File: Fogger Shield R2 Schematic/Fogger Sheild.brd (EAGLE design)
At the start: 53 x 47 mm, 23 parts, among them Q1 MOSFET-NCHANNELFQP30N06L, U1 ARDUINO_SHIELDLABEL

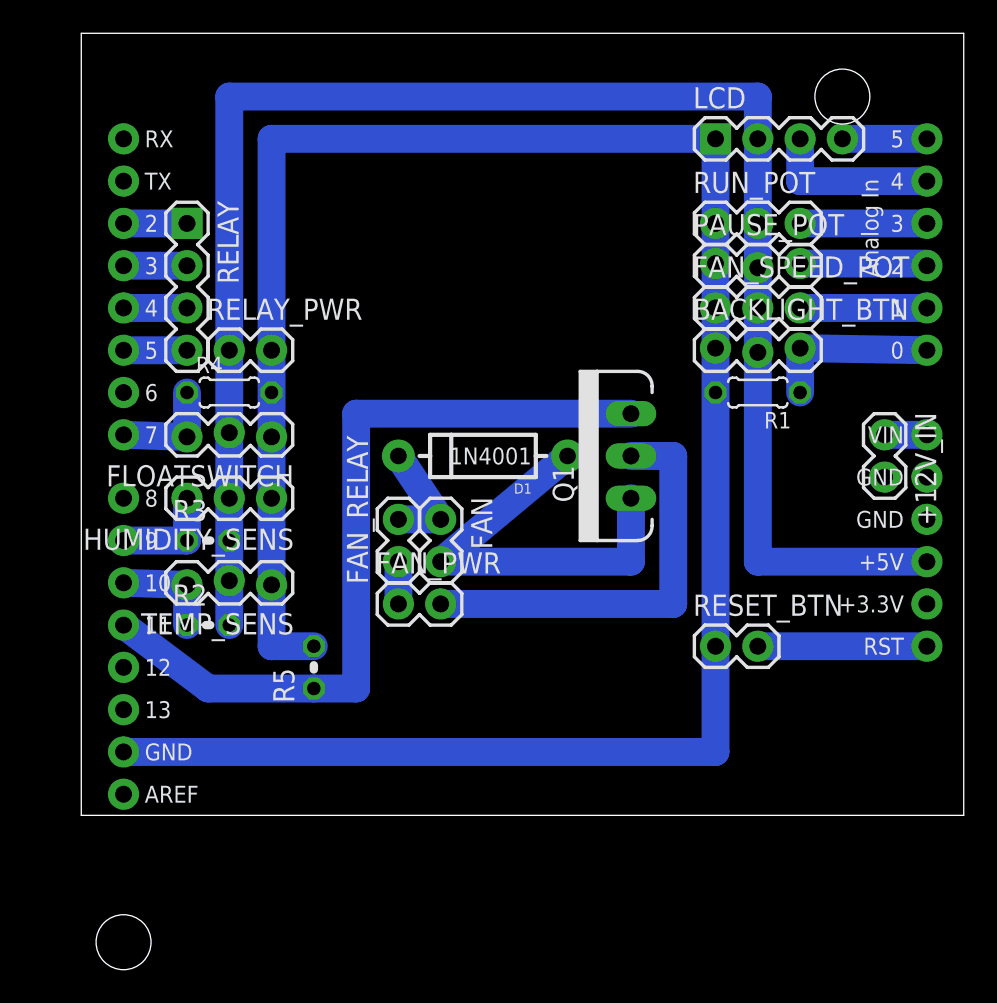
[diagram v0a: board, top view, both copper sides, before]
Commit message: Updated Schematic
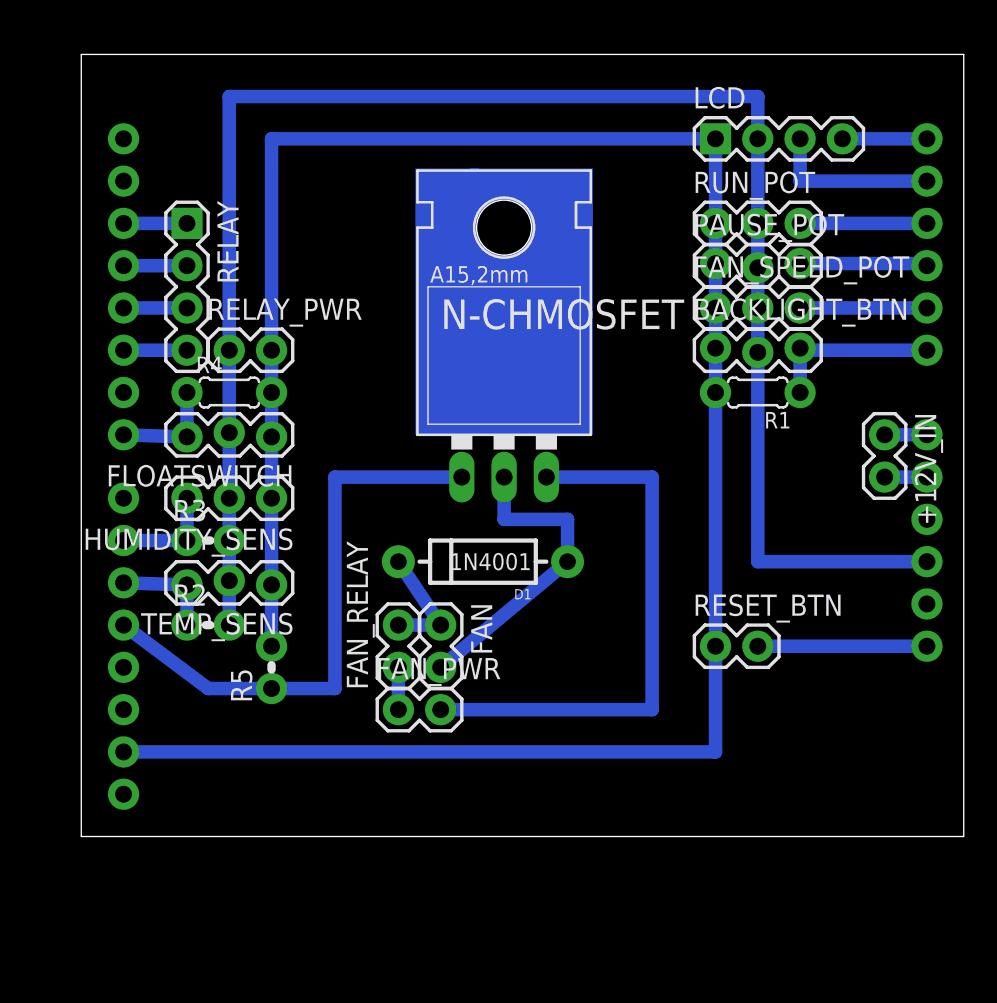
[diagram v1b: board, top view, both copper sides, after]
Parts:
- removed Q1: MOSFET-NCHANNELFQP30N06L, SparkFun-DiscreteSemi:TO220V
- added N-CHMOSFET: V_REG_LD1117VXX, SparkFun-PowerIC:78XXL
- U1: value ARDUINO_SHIELDLABEL -> ARDUINO_SHIELDNO_SILK; device SparkFun-Boards:DUEMILANOVE_SHIELD -> SparkFun-Boards:DUEMILANOVE_VIAS
- moved U1 12.7 mm to (3.81, 34.3)
- moved D1 6.35 mm to (27.9, 50.8)
- moved FAN 6.35 mm to (25.4, 47.0)
- moved FAN_PWR 6.35 mm to (22.9, 41.9)
- moved FAN_RELAY 6.35 mm to (22.9, 44.5)
- moved R5 2.54 mm to (15.2, 44.5)
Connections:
- net N$25: now also N-CHMOSFET.IN; no longer Q1.3
- net N$26: now also N-CHMOSFET.OUT; no longer Q1.2
- net N$27: now also N-CHMOSFET.GND; no longer Q1.1
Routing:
- net N$25: track 48.3 -> 34.3 mm
- net N$26: track 25.4 -> 33.0 mm
- net N$27: track 25.2 -> 18.8 mm
- net N$10: track 0.00 -> 2.54 mm
- net DGND: track 132.2 -> 129.7 mm
